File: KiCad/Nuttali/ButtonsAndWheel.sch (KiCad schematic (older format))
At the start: 17 parts, among them J3 Conn_01x03_Male, SW8 Rotary_Encoder, U6 Button, U7 Button, U8 Scroll_button, U9 Button

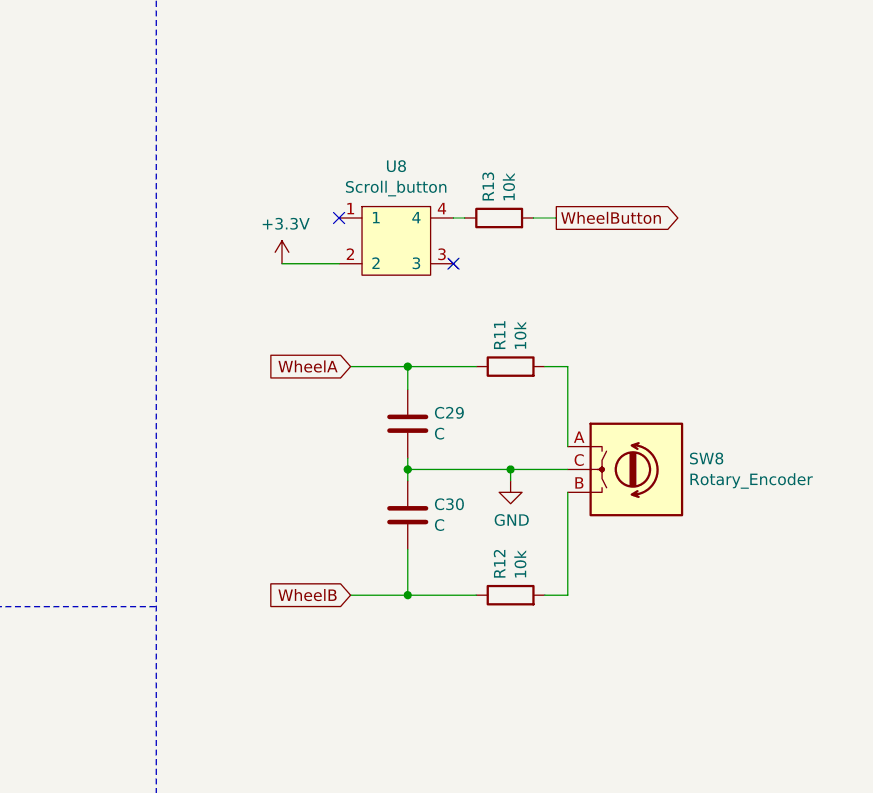
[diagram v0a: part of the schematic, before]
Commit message: Finnished the pcb
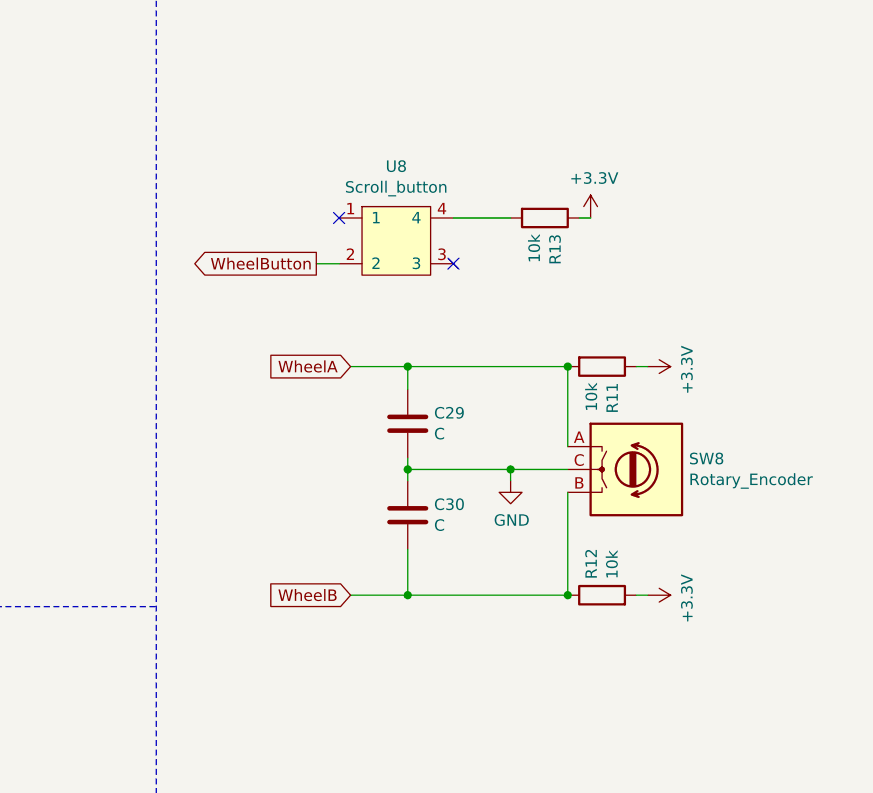
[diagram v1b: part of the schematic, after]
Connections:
- net +3V3: now also R11.1, R12.2, R13.1; no longer U8.2
- net WheelA: now also R11.2, SW8.A; no longer R11.1
- net WheelB: now also SW8.B
- net WheelButton: now also U8.2; no longer R13.2
- net at U8.4: now also R13.2; no longer R13.1
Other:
- moved on the sheet: R11, R12, R13
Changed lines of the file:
@@
 L Nuttali-rescue:+3.3V-power #PWR0148
 U 1 1 602BC22A
-P 3650 2750
-F 0 "#PWR0148" H 3650 2600 50  0001 C CNN
-F 1 "+3.3V" H 3665 2923 50  0000 C CNN
-F 2 "" H 3650 2750 50  0001 C CNN
-F 3 "" H 3650 2750 50  0001 C CNN
-	1    3650 2750
+P 5000 2550
+F 0 "#PWR0148" H 5000 2400 50  0001 C CNN
+F 1 "+3.3V" H 5015 2723 50  0000 C CNN
+F 2 "" H 5000 2550 50  0001 C CNN
+F 3 "" H 5000 2550 50  0001 C CNN
+	1    5000 2550
 	1    0    0    -1
 $EndComp
@@
 L Nuttali-rescue:R-Device R13
 U 1 1 602BC230
-P 4600 2550
-F 0 "R13" H 4670 2596 50  0000 L CNN
-F 1 "10k" H 4670 2505 50  0000 L CNN
-F 2 "Resistor_SMD:R_0805_2012Metric_Pad1.20x1.40mm_HandSolder" V 4530 2550 50  0001 C CNN
-F 3 "~" H 4600 2550 50  0001 C CNN
-	1    4600 2550
-	0    -1   -1   0
-$EndComp
-Wire Wire Line
-	3650 2750 3900 2750
-Wire Wire Line
-	4400 2550 4450 2550
-Wire Wire Line
-	4750 2550 4850 2550
-Text GLabel 4850 2550 2    50   Output ~ 0
+P 4800 2550
+F 0 "R13" H 4870 2596 50  0000 L CNN
+F 1 "10k" H 4870 2505 50  0000 L CNN
+F 2 "Resistor_SMD:R_0805_2012Metric_Pad1.20x1.40mm_HandSolder" V 4730 2550 50  0001 C CNN
+F 3 "~" H 4800 2550 50  0001 C CNN
+	1    4800 2550
+	0    1    1    0
+$EndComp
+Wire Wire Line
+	4400 2550 4650 2550
+Wire Wire Line
+	5000 2550 4950 2550
+Wire Wire Line
+	3900 2750 3800 2750
+Text GLabel 3800 2750 0    50   Output ~ 0
 WheelButton
 $Comp
@@
 L Nuttali-rescue:R-Device R11
 U 1 1 6031998E
-P 4650 3200
-F 0 "R11" H 4720 3246 50  0000 L CNN
-F 1 "10k" H 4720 3155 50  0000 L CNN
-F 2 "Resistor_SMD:R_0805_2012Metric_Pad1.20x1.40mm_HandSolder" V 4580 3200 50  0001 C CNN
-F 3 "~" H 4650 3200 50  0001 C CNN
-	1    4650 3200
-	0    -1   -1   0
+P 5050 3200
+F 0 "R11" H 5120 3246 50  0000 L CNN
+F 1 "10k" H 5120 3155 50  0000 L CNN
+F 2 "Resistor_SMD:R_0805_2012Metric_Pad1.20x1.40mm_HandSolder" V 4980 3200 50  0001 C CNN
+F 3 "~" H 5050 3200 50  0001 C CNN
+	1    5050 3200
+	0    1    1    0
 $EndComp
 $Comp
 L Nuttali-rescue:R-Device R12
 U 1 1 6031A38F
-P 4650 4200
-F 0 "R12" H 4720 4246 50  0000 L CNN
-F 1 "10k" H 4720 4155 50  0000 L CNN
-F 2 "Resistor_SMD:R_0805_2012Metric_Pad1.20x1.40mm_HandSolder" V 4580 4200 50  0001 C CNN
-F 3 "~" H 4650 4200 50  0001 C CNN
-	1    4650 4200
+P 5050 4200
+F 0 "R12" H 5120 4246 50  0000 L CNN
+F 1 "10k" H 5120 4155 50  0000 L CNN
+F 2 "Resistor_SMD:R_0805_2012Metric_Pad1.20x1.40mm_HandSolder" V 4980 4200 50  0001 C CNN
+F 3 "~" H 5050 4200 50  0001 C CNN
+	1    5050 4200
 	0    -1   -1   0
 $EndComp
 Wire Wire Line
 	4900 3550 4900 3200
-Wire Wire Line
-	4900 3200 4800 3200
-Wire Wire Line
-	4500 3200 4200 3200
 Wire Wire Line
 	4200 3200 4200 3300
@@
 Wire Wire Line
 	4900 3750 4900 4200
-Wire Wire Line
-	4900 4200 4800 4200
-Wire Wire Line
-	4500 4200 4200 4200
 Wire Wire Line
 	4200 4200 4200 4000
@@
 Wire Wire Line
 	9350 3400 9350 3850
+Connection ~ 4900 3200
+Wire Wire Line
+	4200 3200 4900 3200
+$Comp
+L Nuttali-rescue:+3.3V-power #PWR0146
+U 1 1 604D0219
+P 5250 3200
+F 0 "#PWR0146" H 5250 3050 50  0001 C CNN
+F 1 "+3.3V" H 5265 3373 50  0000 C CNN
+F 2 "" H 5250 3200 50  0001 C CNN
+F 3 "" H 5250 3200 50  0001 C CNN
+	1    5250 3200
+	0    1    1    0
+$EndComp
+Wire Wire Line
+	5250 3200 5200 3200
+Connection ~ 4900 4200
+Wire Wire Line
+	4200 4200 4900 4200
+$Comp
+L Nuttali-rescue:+3.3V-power #PWR0149
+U 1 1 604D56F4
+P 5250 4200
+F 0 "#PWR0149" H 5250 4050 50  0001 C CNN
+F 1 "+3.3V" H 5265 4373 50  0000 C CNN
+F 2 "" H 5250 4200 50  0001 C CNN
+F 3 "" H 5250 4200 50  0001 C CNN
+	1    5250 4200
+	0    1    1    0
+$EndComp
+Wire Wire Line
+	5250 4200 5200 4200
 $EndSCHEMATC

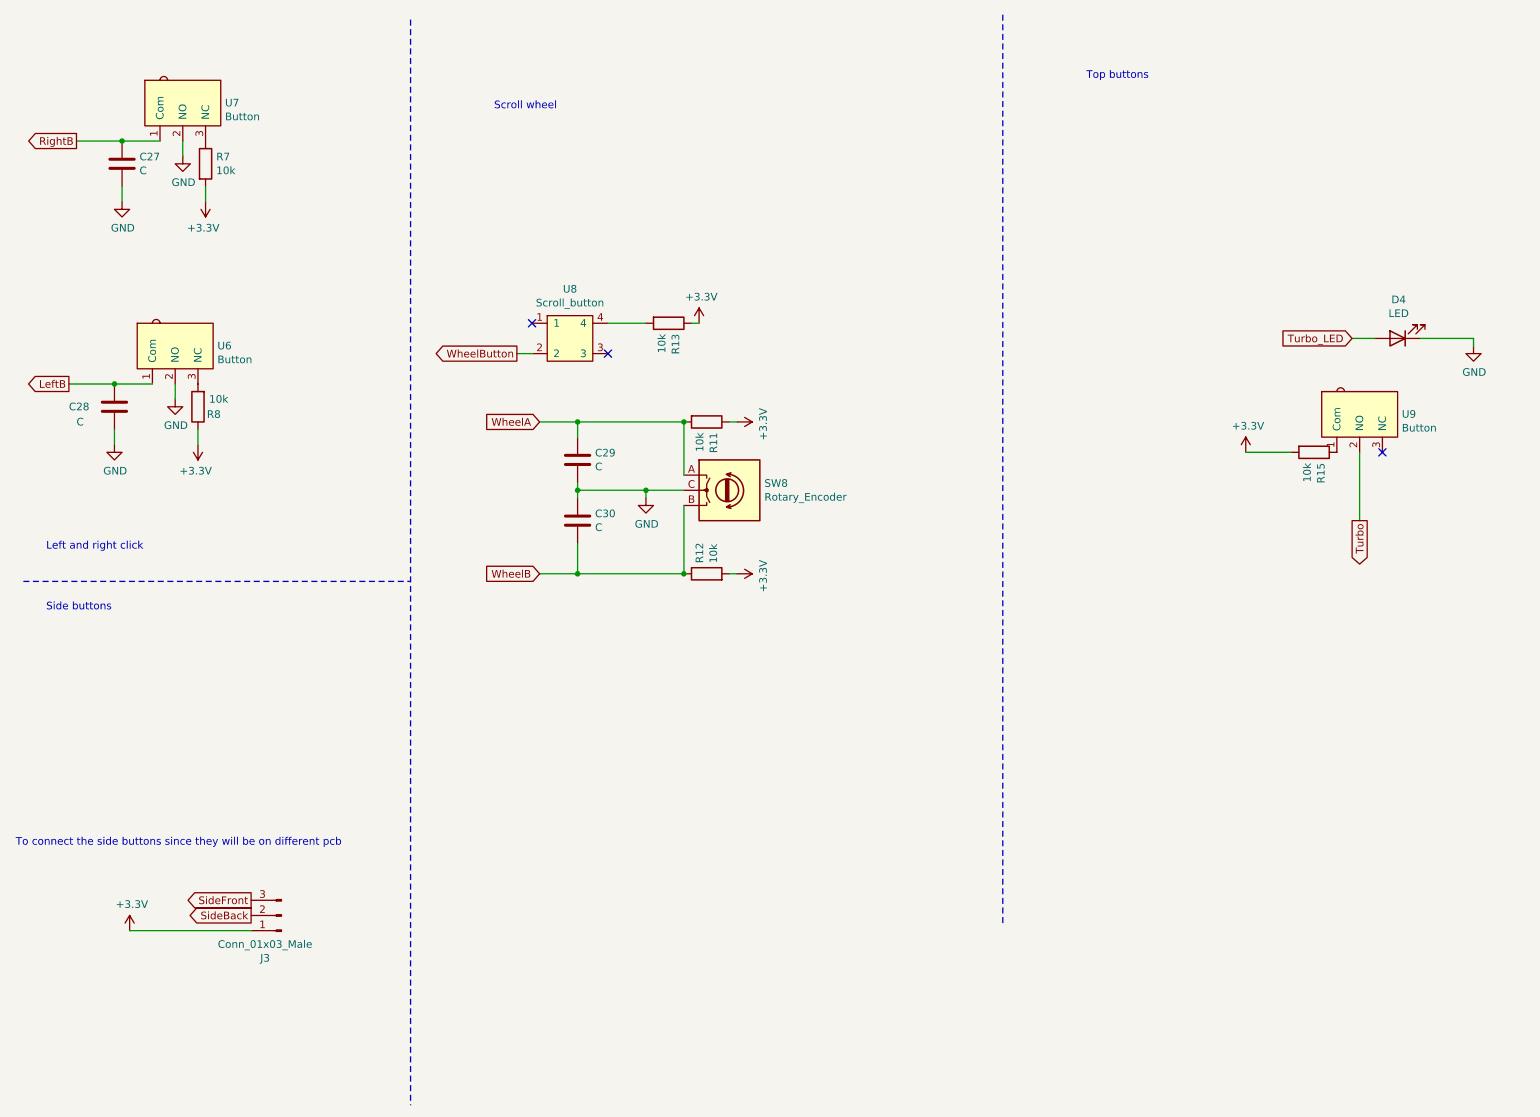
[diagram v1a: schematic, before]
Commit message: Finnished design.
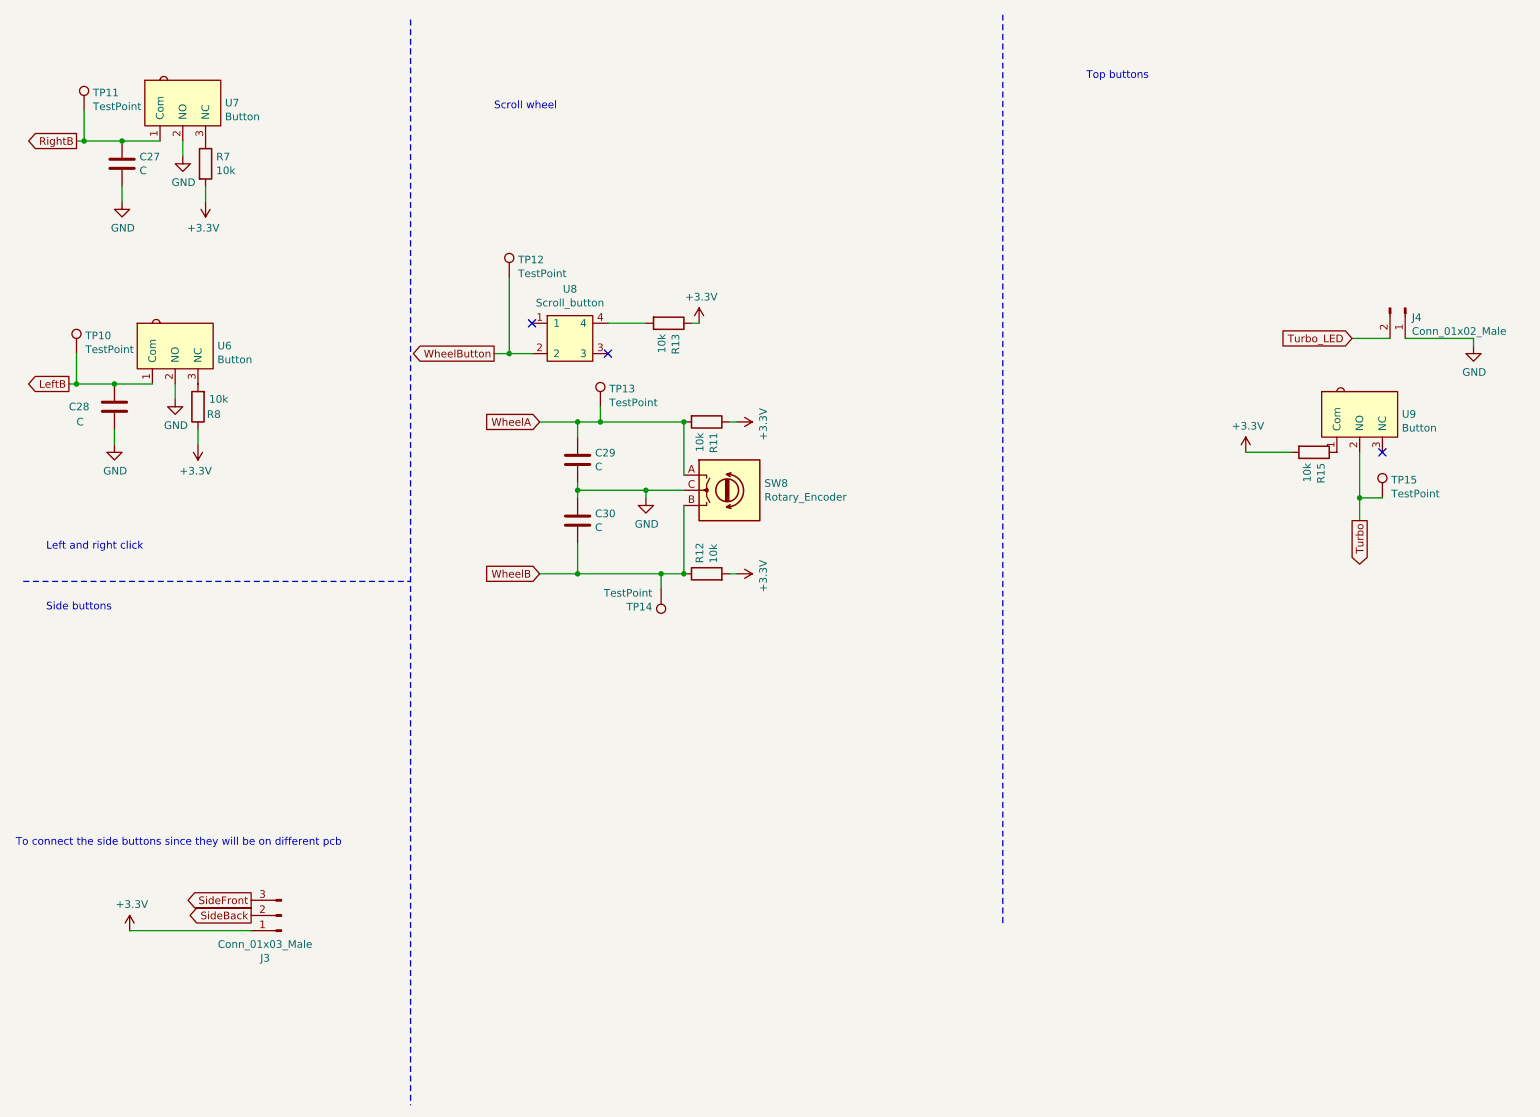
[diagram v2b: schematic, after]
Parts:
- removed D4: LED, Nuttali:LED, symbol Nuttali-rescue:LED-Device
- added J4: Conn_01x02_Male, Connector_PinSocket_2.54mm:PinSocket_1x02_P2.54mm_Vertical, symbol Connector:Conn_01x02_Male
- added TP10, TP11, TP12, TP13, TP14, TP15: TestPoint, TestPoint:TestPoint_Pad_1.0x1.0mm, symbol Nuttali-rescue:TestPoint-Connector
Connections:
- net GND: now also J4.1 (Pin_1)
- net LeftB: now also TP10.1
- net RightB: now also TP11.1
- net Turbo: now also TP15.1
- net Turbo_LED: now also J4.2 (Pin_2)
- net WheelA: now also TP13.1
- net WheelB: now also TP14.1
- net WheelButton: now also TP12.1
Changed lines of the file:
@@
 Wire Wire Line
 	5000 2550 4950 2550
-Wire Wire Line
-	3900 2750 3800 2750
-Text GLabel 3800 2750 0    50   Output ~ 0
+Text GLabel 3650 2750 0    50   Output ~ 0
 WheelButton
 $Comp
@@
 $EndComp
 $Comp
-L Nuttali-rescue:LED-Device D4
-U 1 1 602CBCDE
-P 9600 2650
-F 0 "D4" H 9593 2395 50  0000 C CNN
-F 1 "LED" H 9593 2486 50  0000 C CNN
-F 2 "Nuttali:LED" H 9600 2650 50  0001 C CNN
-F 3 "~" H 9600 2650 50  0001 C CNN
-	1    9600 2650
-	-1   0    0    1
-$EndComp
-$Comp
 L Nuttali-rescue:GND-power #PWR0152
 U 1 1 602CF144
@@
 Text GLabel 9300 2650 0    50   Input ~ 0
 Turbo_LED
-Wire Wire Line
-	9300 2650 9450 2650
-Wire Wire Line
-	9750 2650 10100 2650
 Wire Wire Line
 	10100 2700 10100 2650
@@
 Connection ~ 1150 2950
 Wire Wire Line
-	1150 2950 850  2950
+	1150 2950 900  2950
 $Comp
 L Nuttali-rescue:R-Device R7
@@
 $EndComp
 Wire Wire Line
-	900  1350 1200 1350
+	900  1350 950  1350
 Connection ~ 1200 1350
 Wire Wire Line
@@
 	7000 6500 7000 500
 Wire Wire Line
-	9350 3400 9350 3850
+	9350 3400 9350 3700
 Connection ~ 4900 3200
 Wire Wire Line
-	4200 3200 4900 3200
+	4200 3200 4350 3200
 $Comp
 L Nuttali-rescue:+3.3V-power #PWR0146
@@
 Connection ~ 4900 4200
 Wire Wire Line
-	4200 4200 4900 4200
+	4200 4200 4750 4200
 $Comp
 L Nuttali-rescue:+3.3V-power #PWR0149
@@
 Wire Wire Line
 	5250 4200 5200 4200
+$Comp
+L Nuttali-rescue:TestPoint-Connector TP?
+U 1 1 602996E2
+P 950 1150
+AR Path="/601B1425/602996E2" Ref="TP?"  Part="1"
+AR Path="/6022DC9B/602996E2" Ref="TP11"  Part="1"
+F 0 "TP11" H 1008 1268 50  0000 L CNN
+F 1 "TestPoint" H 1008 1177 50  0000 L CNN
+F 2 "TestPoint:TestPoint_Pad_1.0x1.0mm" H 1150 1150 50  0001 C CNN
+F 3 "~" H 1150 1150 50  0001 C CNN
+	1    950  1150
+	1    0    0    -1
+$EndComp
+$Comp
+L Nuttali-rescue:TestPoint-Connector TP?
+U 1 1 6029A34F
+P 900 2750
+AR Path="/601B1425/6029A34F" Ref="TP?"  Part="1"
+AR Path="/6022DC9B/6029A34F" Ref="TP10"  Part="1"
+F 0 "TP10" H 958 2868 50  0000 L CNN
+F 1 "TestPoint" H 958 2777 50  0000 L CNN
+F 2 "TestPoint:TestPoint_Pad_1.0x1.0mm" H 1100 2750 50  0001 C CNN
+F 3 "~" H 1100 2750 50  0001 C CNN
+	1    900  2750
+	1    0    0    -1
+$EndComp
+$Comp
+L Nuttali-rescue:TestPoint-Connector TP?
+U 1 1 6029B953
+P 3750 2250
+AR Path="/601B1425/6029B953" Ref="TP?"  Part="1"
+AR Path="/6022DC9B/6029B953" Ref="TP12"  Part="1"
+F 0 "TP12" H 3808 2368 50  0000 L CNN
+F 1 "TestPoint" H 3808 2277 50  0000 L CNN
+F 2 "TestPoint:TestPoint_Pad_1.0x1.0mm" H 3950 2250 50  0001 C CNN
+F 3 "~" H 3950 2250 50  0001 C CNN
+	1    3750 2250
+	1    0    0    -1
+$EndComp
+$Comp
+L Nuttali-rescue:TestPoint-Connector TP?
+U 1 1 6029C224
+P 4350 3100
+AR Path="/601B1425/6029C224" Ref="TP?"  Part="1"
+AR Path="/6022DC9B/6029C224" Ref="TP13"  Part="1"
+F 0 "TP13" H 4408 3218 50  0000 L CNN
+F 1 "TestPoint" H 4408 3127 50  0000 L CNN
+F 2 "TestPoint:TestPoint_Pad_1.0x1.0mm" H 4550 3100 50  0001 C CNN
+F 3 "~" H 4550 3100 50  0001 C CNN
+	1    4350 3100
+	1    0    0    -1
+$EndComp
+$Comp
+L Nuttali-rescue:TestPoint-Connector TP?
+U 1 1 6029CEB2
+P 4750 4300
+AR Path="/601B1425/6029CEB2" Ref="TP?"  Part="1"
+AR Path="/6022DC9B/6029CEB2" Ref="TP14"  Part="1"
+F 0 "TP14" H 4808 4418 50  0000 L CNN
+F 1 "TestPoint" H 4808 4327 50  0000 L CNN
+F 2 "TestPoint:TestPoint_Pad_1.0x1.0mm" H 4950 4300 50  0001 C CNN
+F 3 "~" H 4950 4300 50  0001 C CNN
+	1    4750 4300
+	-1   0    0    1
+$EndComp
+$Comp
+L Nuttali-rescue:TestPoint-Connector TP?
+U 1 1 6029F887
+P 9500 3700
+AR Path="/601B1425/6029F887" Ref="TP?"  Part="1"
+AR Path="/6022DC9B/6029F887" Ref="TP15"  Part="1"
+F 0 "TP15" H 9558 3818 50  0000 L CNN
+F 1 "TestPoint" H 9558 3727 50  0000 L CNN
+F 2 "TestPoint:TestPoint_Pad_1.0x1.0mm" H 9700 3700 50  0001 C CNN
+F 3 "~" H 9700 3700 50  0001 C CNN
+	1    9500 3700
+	1    0    0    -1
+$EndComp
+Wire Wire Line
+	9500 3700 9350 3700
+Connection ~ 9350 3700
+Wire Wire Line
+	9350 3700 9350 3850
+Wire Wire Line
+	900  2950 900  2750
+Connection ~ 900  2950
+Wire Wire Line
+	900  2950 850  2950
+Wire Wire Line
+	950  1350 950  1150
+Connection ~ 950  1350
+Wire Wire Line
+	950  1350 1200 1350
+Wire Wire Line
+	3650 2750 3750 2750
+Wire Wire Line
+	3750 2250 3750 2750
+Connection ~ 3750 2750
+Wire Wire Line
+	3750 2750 3900 2750
+$Comp
+L Connector:Conn_01x02_Male J4
+U 1 1 602CAADB
+P 9650 2450
+F 0 "J4" V 9712 2494 50  0000 L CNN
+F 1 "Conn_01x02_Male" V 9803 2494 50  0000 L CNN
+F 2 "Connector_PinSocket_2.54mm:PinSocket_1x02_P2.54mm_Vertical" H 9650 2450 50  0001 C CNN
+F 3 "~" H 9650 2450 50  0001 C CNN
+	1    9650 2450
+	0    1    1    0
+$EndComp
+Wire Wire Line
+	9650 2650 10100 2650
+Wire Wire Line
+	9300 2650 9550 2650
+Wire Wire Line
+	4350 3100 4350 3200
+Connection ~ 4350 3200
+Wire Wire Line
+	4350 3200 4900 3200
+Wire Wire Line
+	4750 4300 4750 4200
+Connection ~ 4750 4200
+Wire Wire Line
+	4750 4200 4900 4200
 $EndSCHEMATC
